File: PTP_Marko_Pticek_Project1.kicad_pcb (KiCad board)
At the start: 2 copper layers, 45 parts, among them J1 Screw_Terminal_01x02, SW1 SW_Push, SW2 SW_Wuerth_450301014042, U1 LM2574N-5, U2 4027, U3 4027, U4 74LS47, U5 HDSP-7401, U6 74LVC1G11, U7 NE555P

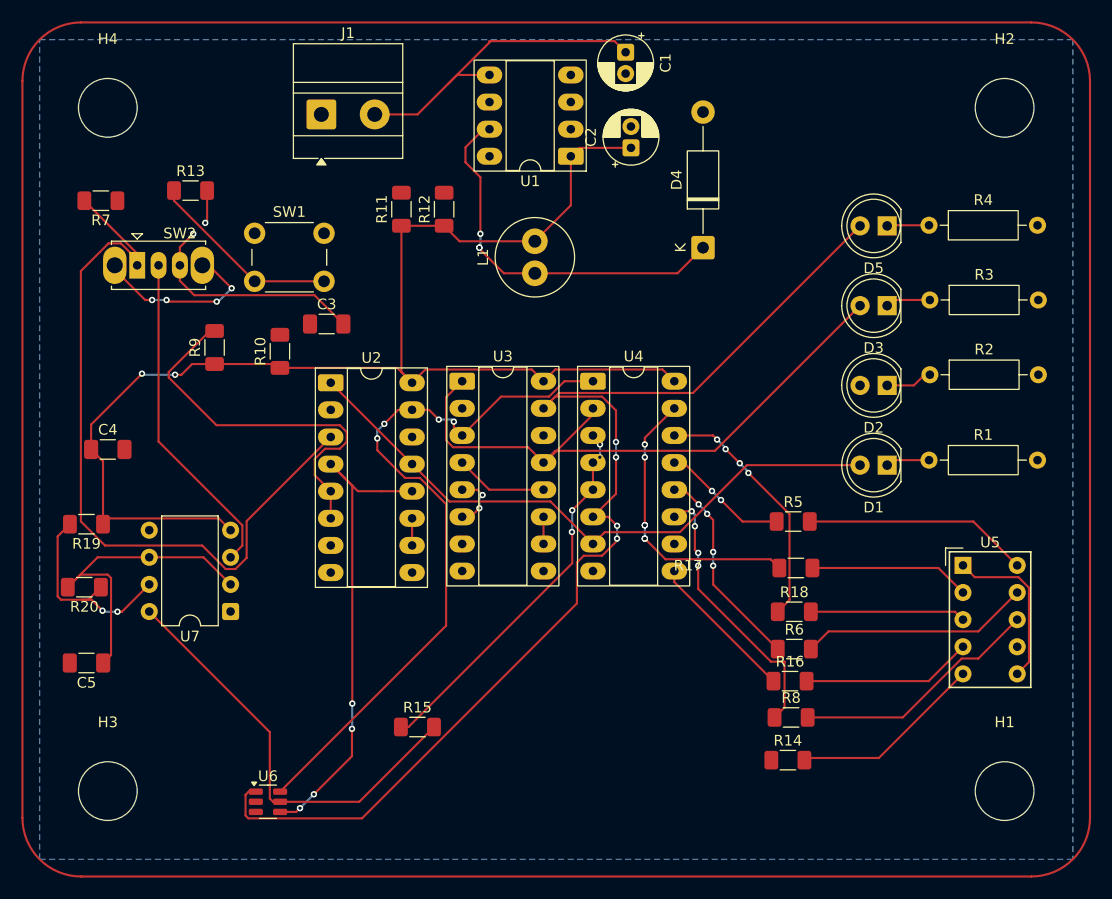
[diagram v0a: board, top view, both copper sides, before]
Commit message: dovrsavanje
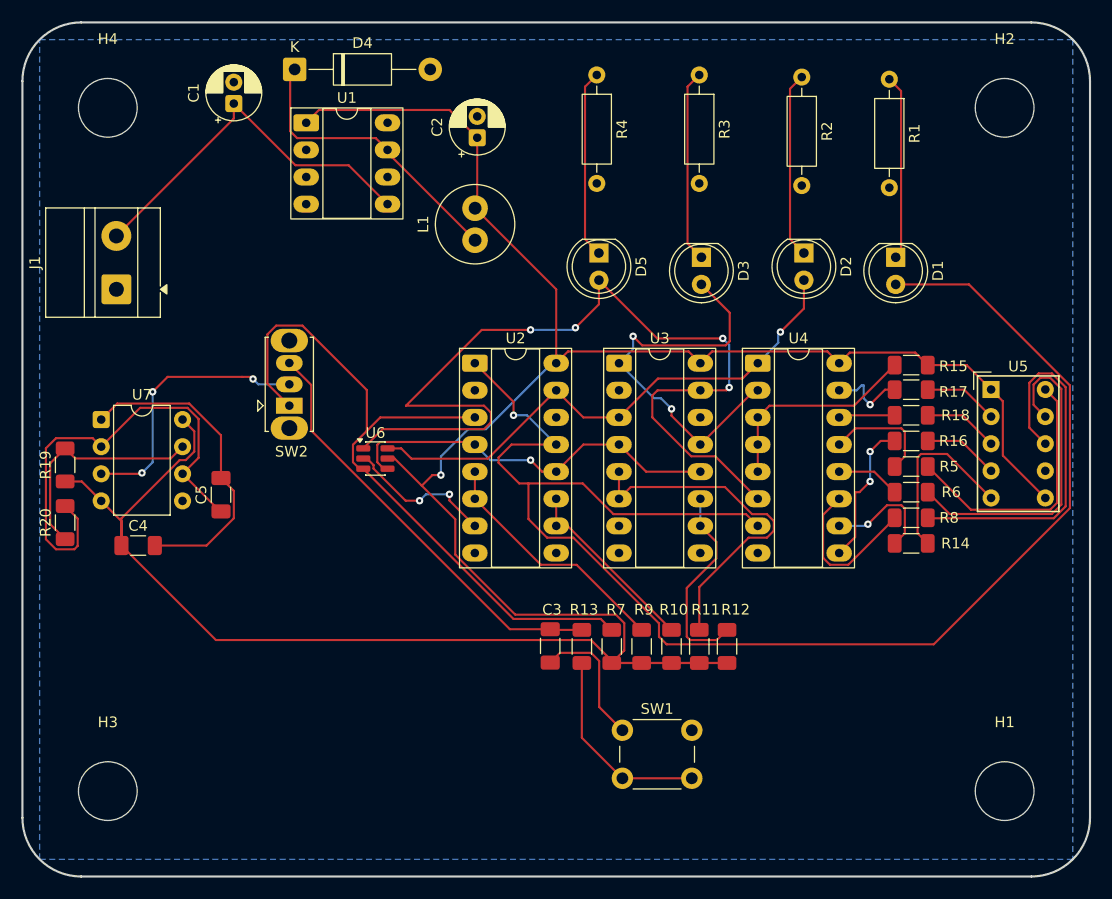
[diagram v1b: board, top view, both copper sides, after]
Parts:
- moved R7 63.5 mm to (161.2, 113.5), turned to 90 degrees
- moved SW1 57.9 mm to (162.2, 121.3)
- moved R15 57.3 mm to (189.2, 87.1)
- moved R13 56.3 mm to (158.4, 113.5), turned to 90 degrees
- moved R11 49.6 mm to (169.4, 113.5)
- moved R9 48.8 mm to (164.0, 113.5)
- moved R12 48.8 mm to (172.0, 113.5)
- moved R10 45.9 mm to (166.8, 113.5)
- moved D4 41.7 mm to (131.5, 59.4), turned to 0 degrees
- moved C1 37.0 mm to (125.8, 62.6), turned to 90 degrees
- moved C3 36.7 mm to (155.4, 113.4), turned to 90 degrees
- moved R1 35.9 mm to (187.2, 60.3), turned to -90 degrees
- moved R4 34.2 mm to (159.8, 59.9), turned to -90 degrees
- moved U6 33.7 mm to (139.1, 95.8)
- moved R2 30.4 mm to (179.0, 60.1), turned to -90 degrees
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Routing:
- net Q0: track 58.9 -> 141.3 mm, vias 0 -> 1
- net +5V: track 181.8 -> 248.3 mm, vias 2 -> 1
- net GND: track 0.00 -> 56.9 mm, vias 0 -> 2
- net Net-(U3A-J): track 5.42 -> 32.9 mm, vias 2 -> 0
- net Q3: track 110.4 -> 87.7 mm
- net Q2: track 59.0 -> 37.7 mm, vias 0 -> 2
- net Net-(U4-f): track 27.1 -> 7.42 mm, vias 6 -> 1
- net Net-(U4-g): track 23.6 -> 5.28 mm, vias 4 -> 0
- net RESET: track 54.4 -> 36.5 mm, vias 4 -> 1
- net Q1: track 68.1 -> 50.5 mm, vias 4 -> 1
- net (no net): track 16.8 -> 0.00 mm, vias 4 -> 0
- net Net-(U3B-J): track 2.54 -> 19.0 mm
- net Net-(U4-BI): track 35.8 -> 19.9 mm, vias 4 -> 0
- net Net-(SW2-A): track 25.0 -> 40.3 mm, vias 2 -> 0
- net Net-(U2B-J): track 2.54 -> 17.4 mm
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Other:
- board outline added: 100 x 80 mm
